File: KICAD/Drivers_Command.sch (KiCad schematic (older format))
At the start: 13 parts, among them U4 CD4053BM96, U5 CD4053BM96, U6 4011

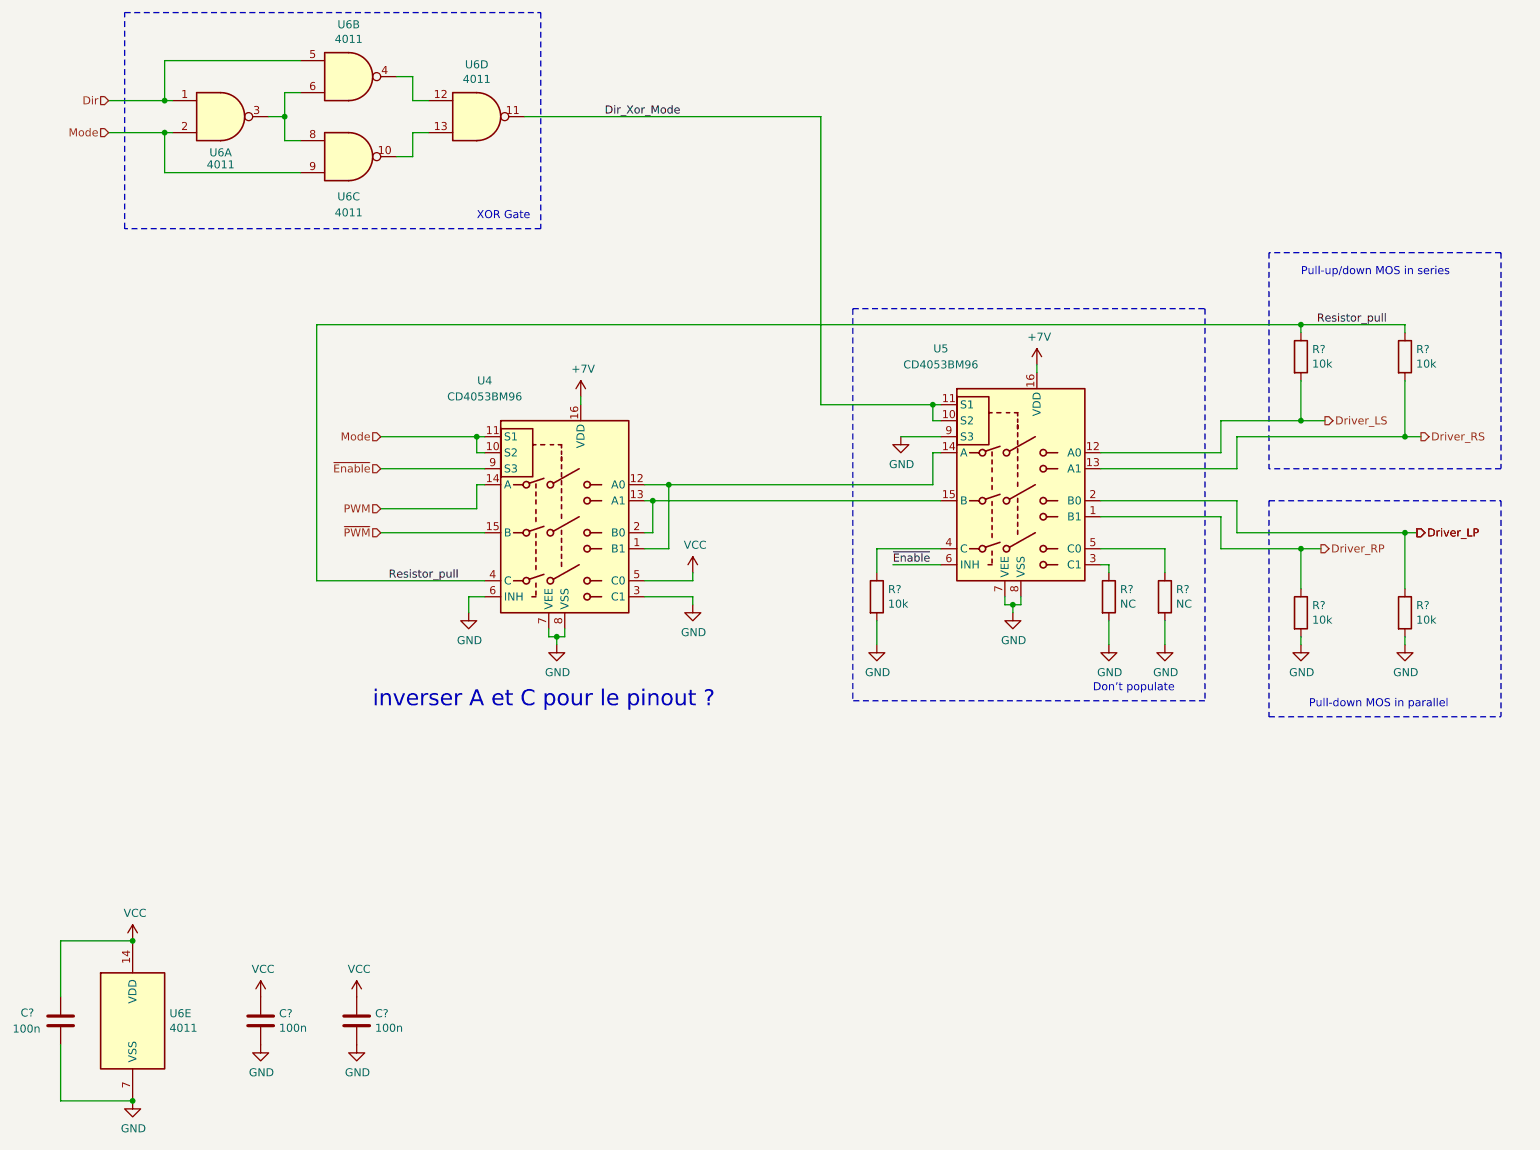
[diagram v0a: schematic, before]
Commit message: minor cleanup
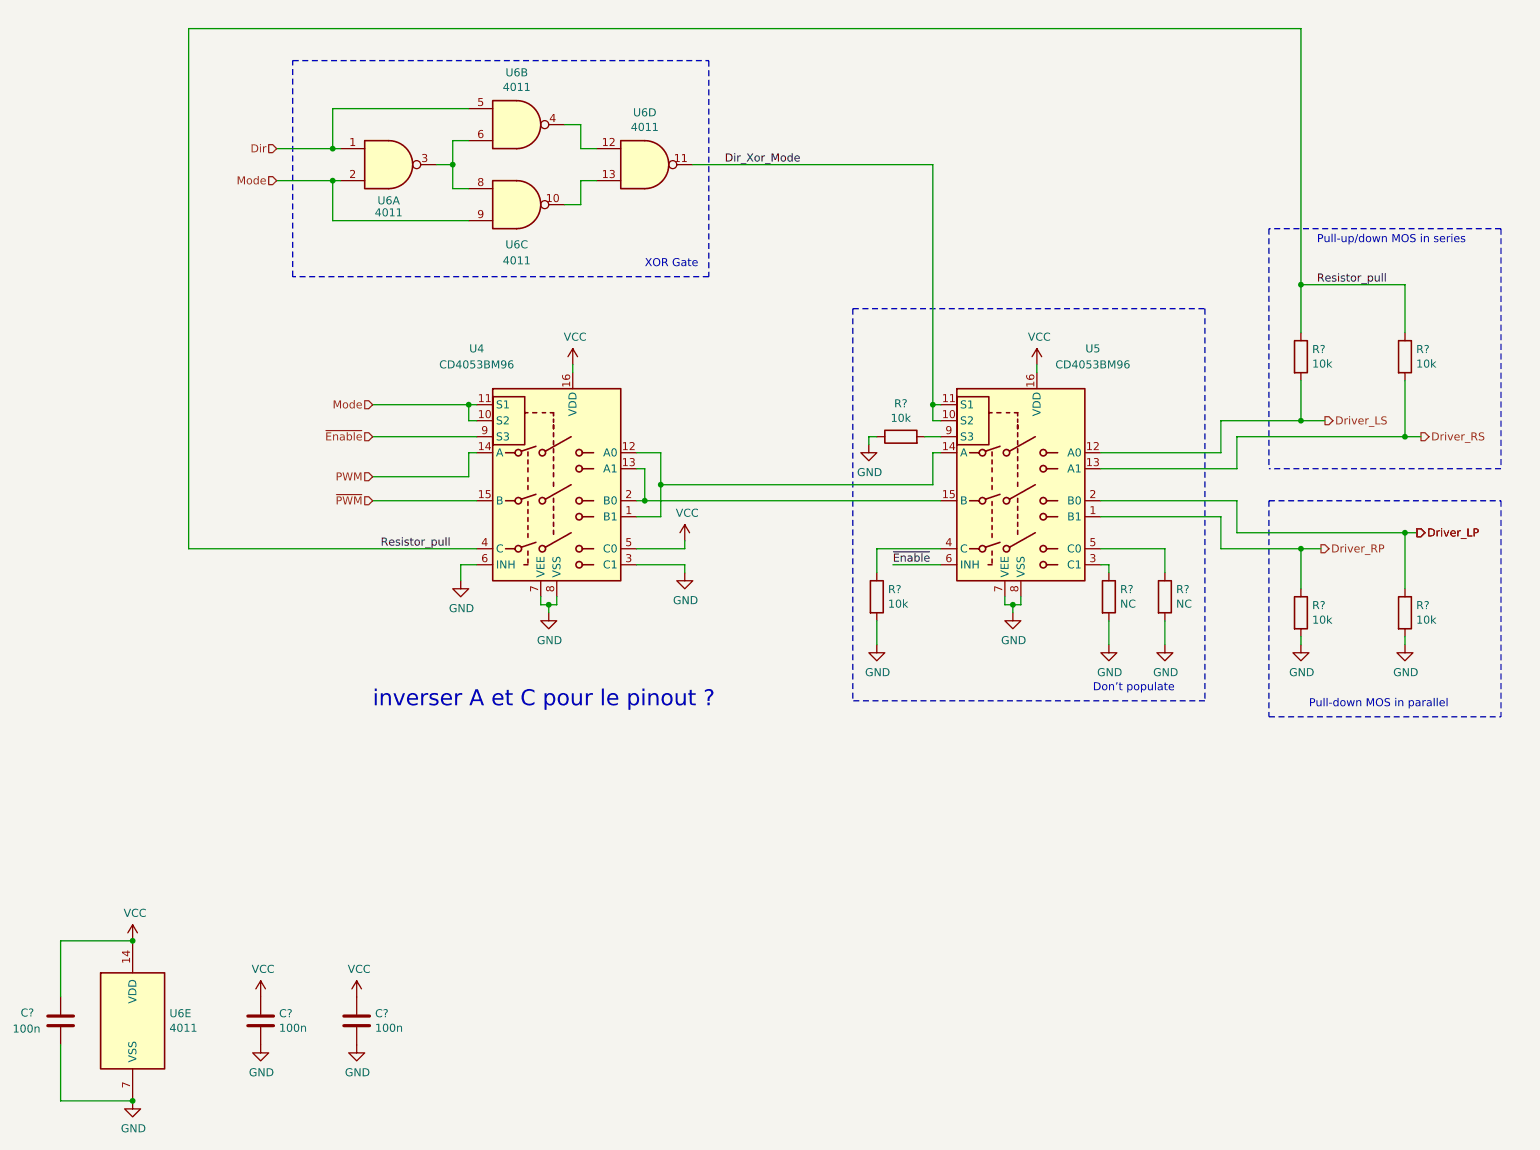
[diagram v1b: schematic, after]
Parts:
- added R?: 10k, Resistor_SMD:R_0805_2012Metric_Pad1.15x1.40mm_HandSolder, symbol Device:R
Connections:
- net +7V is gone; now on net VCC: U4.16 (VDD), U5.16 (VDD)
- net GND: now also R?.1; no longer U5.9 (S3)
- new net: R?.2, U5.9 (S3)
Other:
- moved on the sheet: U4, U6A, U6B, U6C, U6D
